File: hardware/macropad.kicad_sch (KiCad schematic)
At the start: 21 parts, among them J1 Conn_01x04, J2 Conn_01x06, SW1 SW_Push, SW10 RotaryEncoder_Switch, SW2 SW_Push, SW3 SW_Push, SW4 SW_Push, SW5 SW_Push, SW6 SW_Push, SW7 SW_Push, SW8 SW_Push, SW9 SW_Push

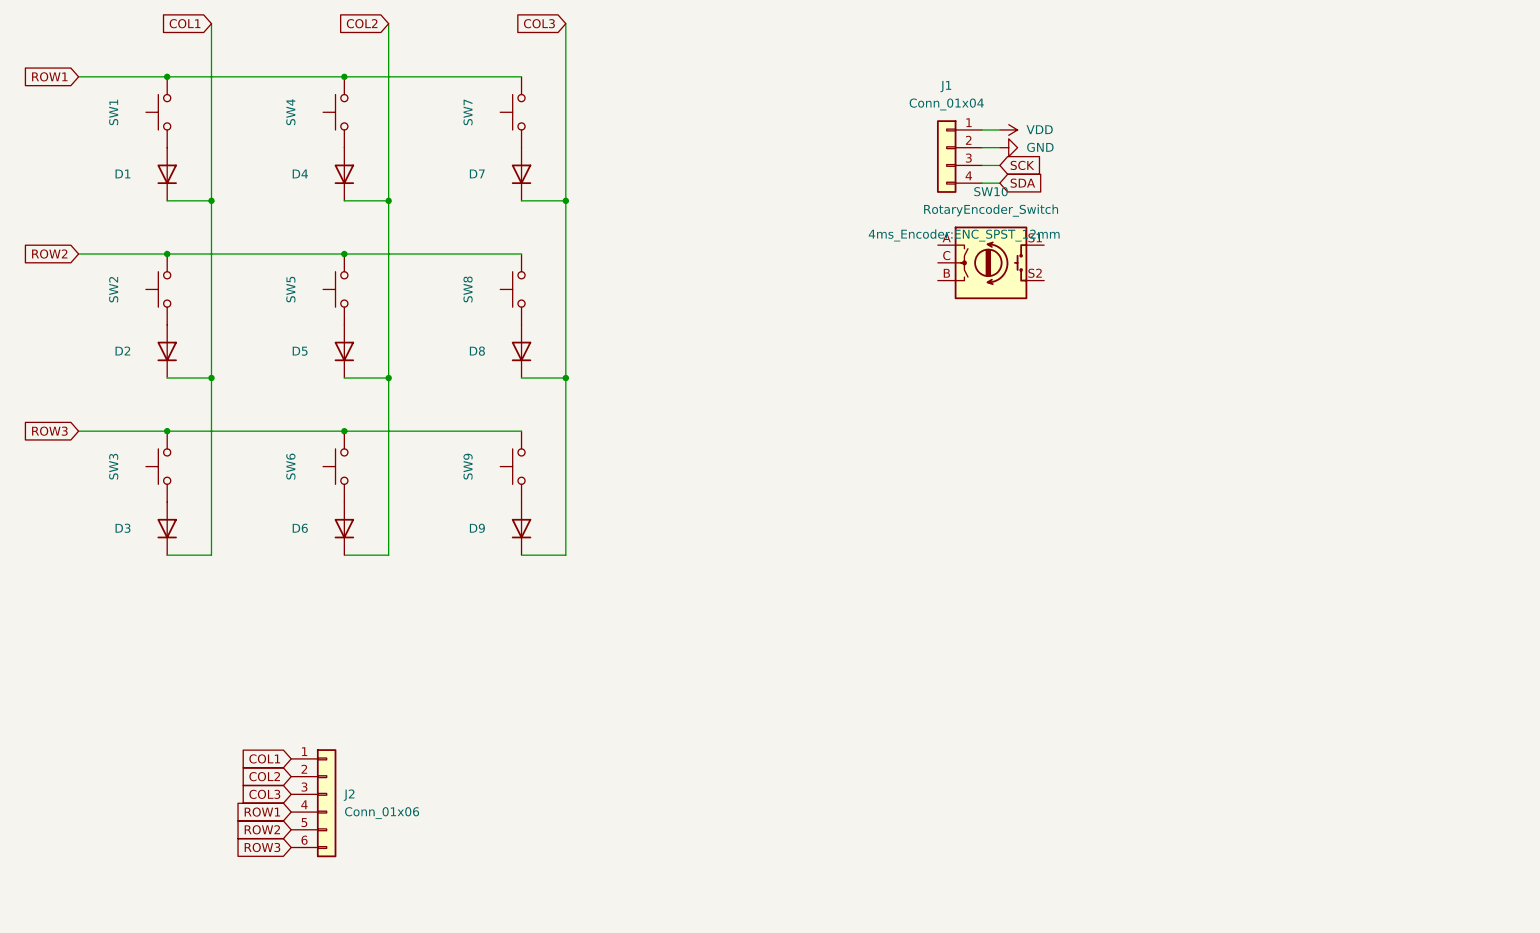
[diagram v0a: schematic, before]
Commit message: :sparkles: Add pico & screen
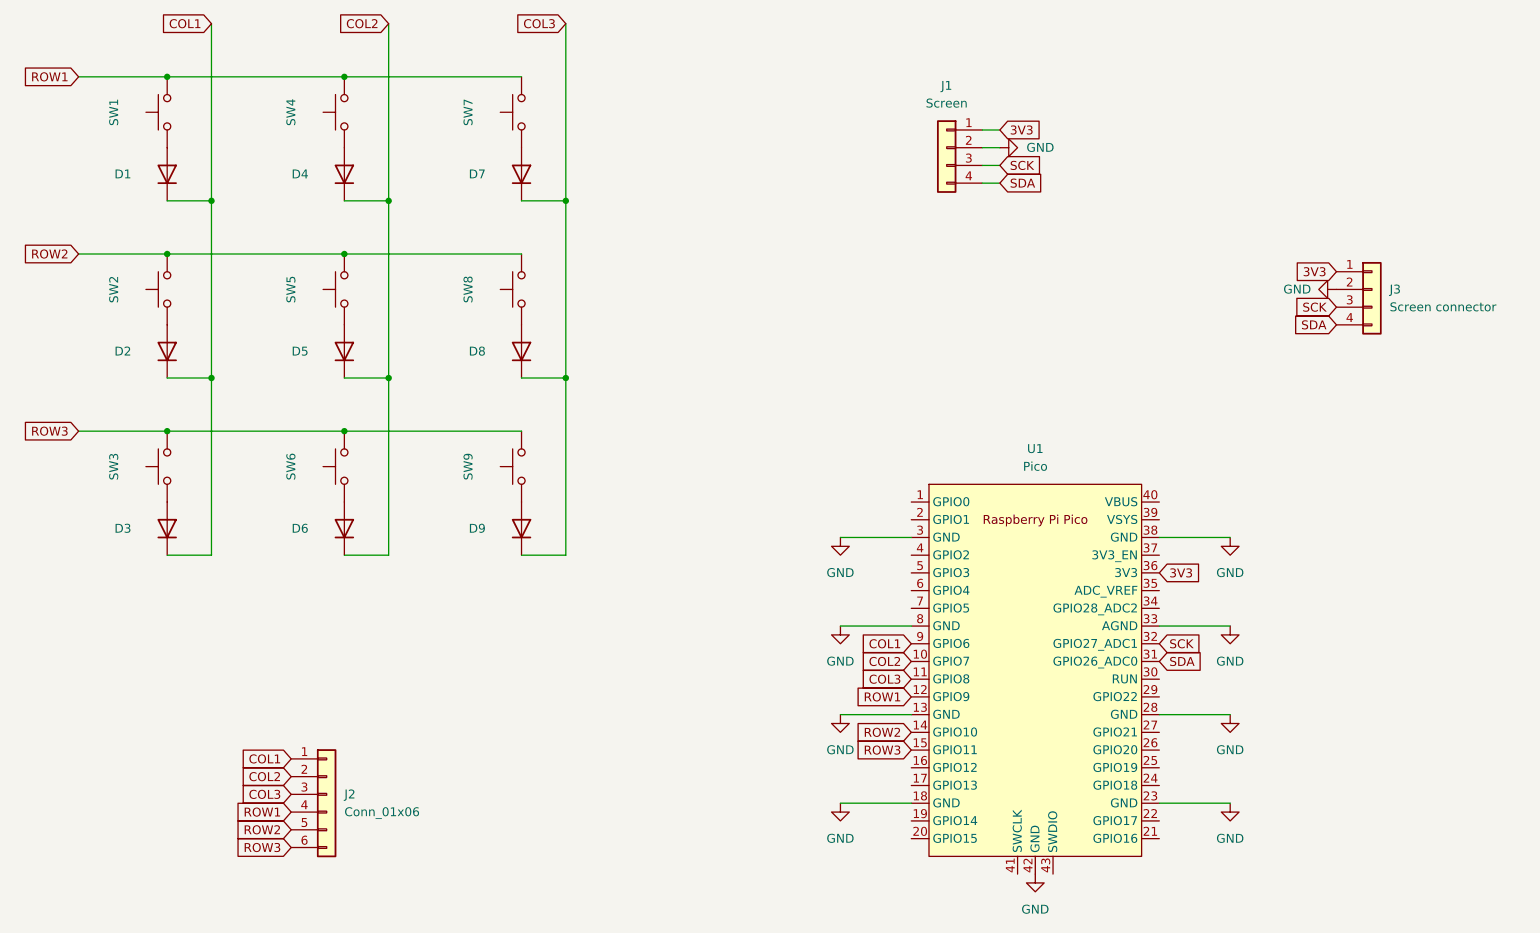
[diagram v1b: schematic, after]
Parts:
- removed SW10: RotaryEncoder_Switch, 4ms_Encoder:ENC_SPST_12mm, symbol Device:RotaryEncoder_Switch
- added J3: Screen connector, Connector_PinHeader_2.54mm:PinHeader_1x04_P2.54mm_Vertical, symbol Connector_Generic:Conn_01x04
- added U1: Pico, MCU_RaspberryPi_and_Boards:RPi_Pico_SMD_TH, symbol MCU_RaspberryPi_and_Boards:Pico
- J1: value Conn_01x04 -> Screen
- J2: footprint Connector_PinHeader_2.54mm:PinHeader_1x06_P2.54mm_Horizontal -> Connector_PinHeader_2.54mm:PinHeader_1x06_P2.54mm_Vertical
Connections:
- net COL1: now also U1.9 (GPIO6)
- net COL2: now also U1.10 (GPIO7)
- net COL3: now also U1.11 (GPIO8)
- net GND: now also J3.2 (Pin_2), U1.13 (GND), U1.18 (GND), U1.23 (GND), U1.28 (GND), U1.3 (GND), U1.33 (AGND), U1.38 (GND), U1.42 (GND), U1.8 (GND)
- net ROW1: now also U1.12 (GPIO9)
- net ROW2: now also U1.14 (GPIO10)
- net ROW3: now also U1.15 (GPIO11)
- net SCK: now also J3.3 (Pin_3), U1.32 (GPIO27_ADC1)
- net SDA: now also J3.4 (Pin_4), U1.31 (GPIO26_ADC0)
- net VDD renamed 3V3
- net 3V3: now also J3.1 (Pin_1), U1.36 (3V3)
